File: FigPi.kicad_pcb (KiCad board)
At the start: 2 copper layers, 25.8 x 40.4 mm, 45 parts, among them J1 MOLEX_47346-100147346, J2 SPI0 / PWM2 / PWM3, J3 UART0 / PWM3 / PWM4, J4 STEMMA_1/QWIIC_1/I2C1/PMW1, J5 ADC / PWM5 / PWM6, J6 STEMMA_0/QWIIC_0/I2C0/PMW0, J7 PWR, SW1 KMS233GLFG, SW2 KMS233GLFG, U1 RP2040, U2 QSPI NOR FLASH 2MiB 2x3mm USO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, U3 AP2112K-3.3, U4 KC2520Z

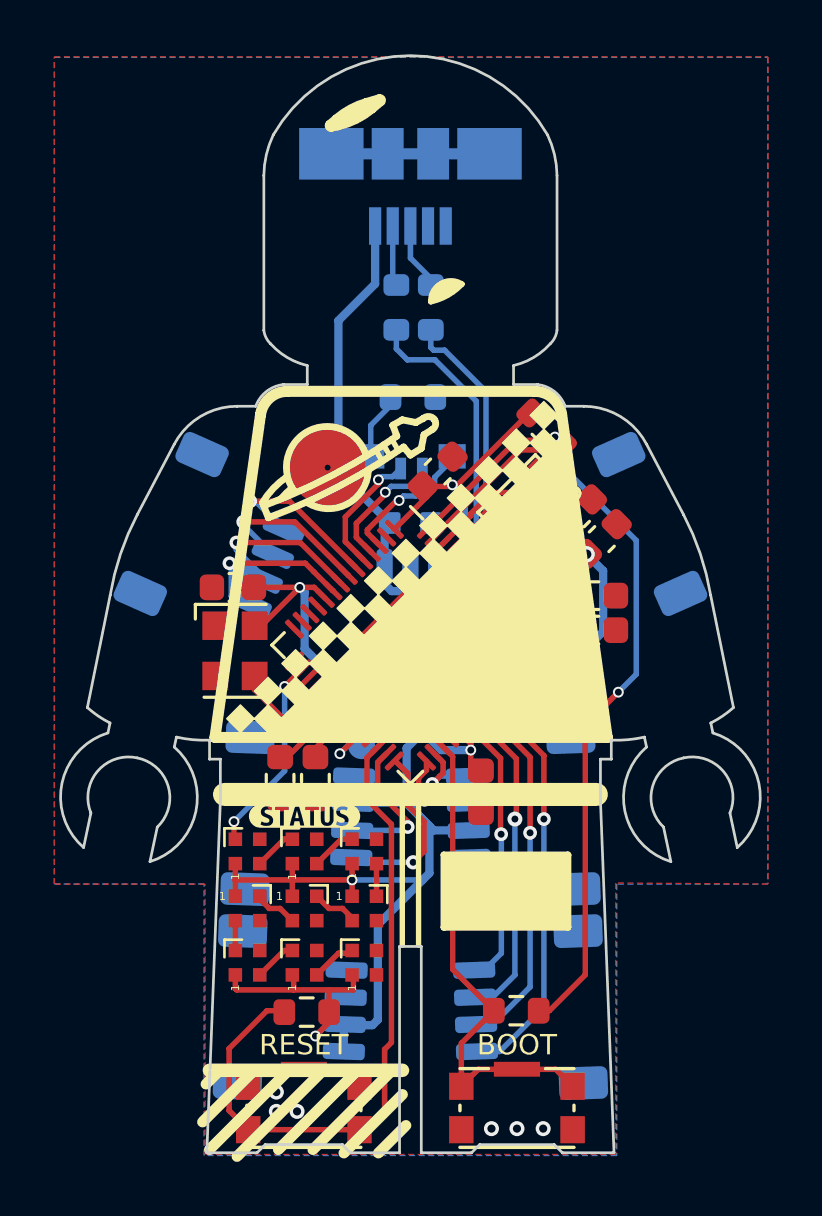
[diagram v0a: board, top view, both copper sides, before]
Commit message: 1.6 - Minor Cosmetic Changes
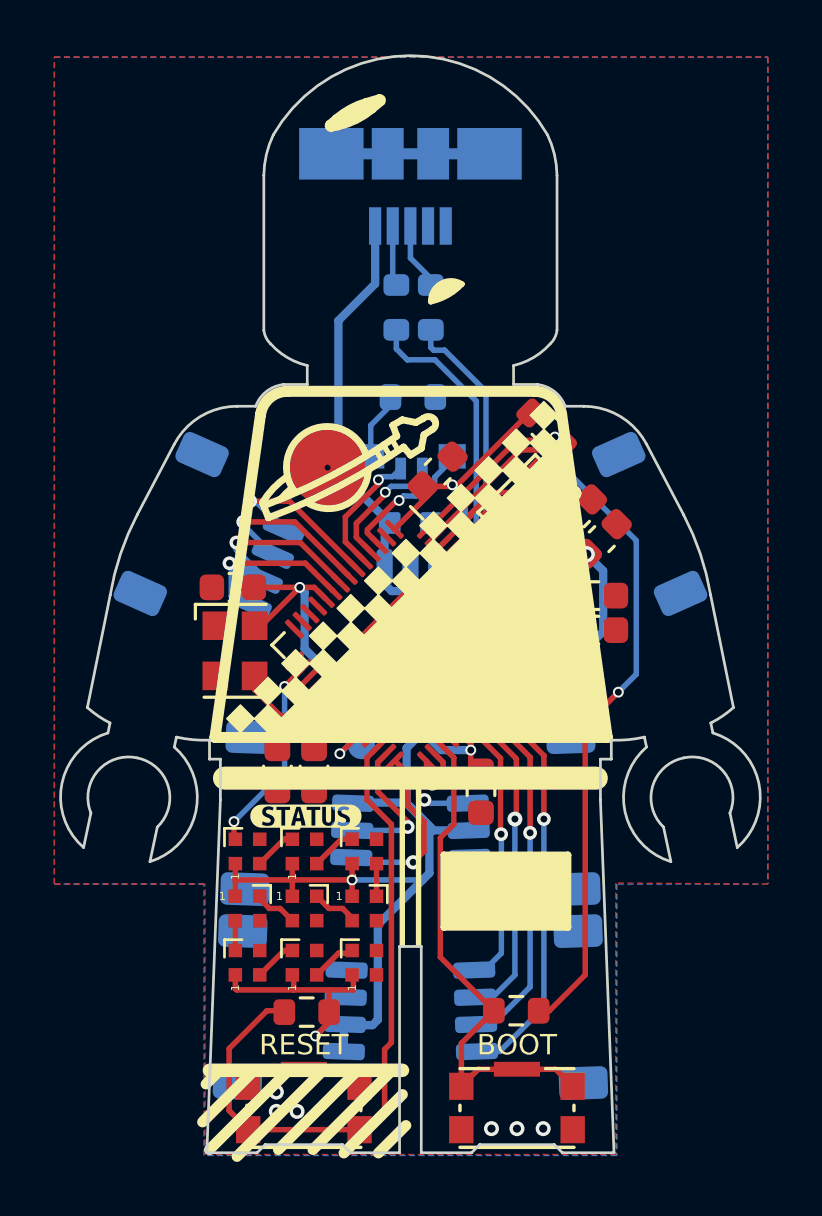
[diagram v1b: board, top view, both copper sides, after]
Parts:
- moved C8 0.32 mm to (7.10, -14.1)
- moved C3 0.30 mm to (8.45, -14.1)
- moved kibuzzard-620D4CA4 0.05 mm to (8.15, -12.4)
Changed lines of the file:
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@@
   )
   (footprint "Capacitor_SMD:C_0603_1608Metric" (layer "F.Cu")
-    (at 7.2 -13.8 90)
+    (at 7.1 -14.1 90)
     (descr "Capacitor SMD 0603 (1608 Metric), square (rectangular) end terminal, IPC_7351 nominal, (Body size source: IPC-SM-782 page 76, https://www.pcb-3d.com/wordpress/wp-content/uploads/ipc-sm-782a_amendment_1_and_2.pdf), generated with kicad-footprint-generator")
     (tags "capacitor")
@@
   )
   (footprint "Capacitor_SMD:C_0603_1608Metric" (layer "F.Cu")
-    (at 8.5 -13.8 90)
+    (at 8.45 -14.1 90)
     (descr "Capacitor SMD 0603 (1608 Metric), square (rectangular) end terminal, IPC_7351 nominal, (Body size source: IPC-SM-782 page 76, https://www.pcb-3d.com/wordpress/wp-content/uploads/ipc-sm-782a_amendment_1_and_2.pdf), generated with kicad-footprint-generator")
     (tags "capacitor")
@@
   )
   (footprint "kibuzzard-620D4CA4" (layer "F.Cu")
-    (at 8.1 -12.4)
+    (at 8.15 -12.4)
     (descr "Converted using: scripting")
     (tags "svg2mod")
@@
   (gr_line (start 11.7 -13.35) (end 11.7 -7.65) (layer "F.SilkS") (width 0.2))
   (gr_arc (start 6.478558 -27.189797) (mid 6.812918 -27.804917) (end 7.46874 -28.05) (layer "F.SilkS") (width 0.4064))
-  (gr_line (start 18.85 -13.2) (end 5.15 -13.2) (layer "F.SilkS") (width 0.85))
+  (gr_line (start 18.85 -13.8) (end 5.15 -13.8) (layer "F.SilkS") (width 0.85))
   (gr_line (start 16.581259 -28.05) (end 7.46874 -28.05) (layer "F.SilkS") (width 0.4064))
   (gr_arc (start 16.581257 -28.05) (mid 17.23708 -27.804917) (end 17.57144 -27.189796) (layer "F.SilkS") (width 0.4064))
@@
   (segment (start 5.55 -6.05) (end 5.55 -6.55) (width 0.2032) (layer "F.Cu") (net 3))
   (segment (start 18.021 -18.679) (end 18.021 -19.2532) (width 0.3048) (layer "F.Cu") (net 3))
+  (segment (start 7.1 -14.875) (end 7.925 -15.7) (width 0.2032) (layer "F.Cu") (net 3))
   (segment (start 9.0038 -5.9962) (end 9 -6) (width 0.2032) (layer "F.Cu") (net 3))
   (segment (start 18.3 -18.4) (end 18.177208 -18.277208) (width 0.3048) (layer "F.Cu") (net 3))
+  (segment (start 7.925 -15.7) (end 8.9 -15.7) (width 0.2032) (layer "F.Cu") (net 3))
   (segment (start 9.282843 -15.7) (end 9.710742 -16.127899) (width 0.2032) (layer "F.Cu") (net 3))
   (segment (start 18.021 -18.964616) (end 17.333592 -18.277208) (width 0.2032) (layer "F.Cu") (net 3))
-  (segment (start 8.9 -15.7) (end 8.591 -15.7) (width 0.2032) (layer "F.Cu") (net 3))
   (segment (start 18.021 -20.5232) (end 18.454002 -20.090198) (width 0.2032) (layer "F.Cu") (net 3))
   (segment (start 7.65 -10.15) (end 7.65 -10.75) (width 0.2032) (layer "F.Cu") (net 3))
@@
   (segment (start 9.9 -6.5) (end 9.9 -6) (width 0.2032) (layer "F.Cu") (net 3))
   (segment (start 17.500155 -20.5232) (end 18.021 -20.5232) (width 0.2032) (layer "F.Cu") (net 3))
-  (segment (start 8.591 -15.7) (end 7.493 -14.602) (width 0.2032) (layer "F.Cu") (net 3))
   (segment (start 17.075658 -22.005596) (end 18.249588 -22.005596) (width 0.2032) (layer "F.Cu") (net 3))
   (segment (start 15.986314 -19.575045) (end 16.269157 -19.292202) (width 0.2032) (layer "F.Cu") (net 3))
@@
   (segment (start 13.875 -2.45) (end 13.85 -2.45) (width 0.2032) (layer "F.Cu") (net 28))
   (segment (start 14.5 -3.075) (end 13.875 -2.45) (width 0.2032) (layer "F.Cu") (net 28))
-  (segment (start 13.559081 -6.748719) (end 15.0754 -5.2324) (width 0.2) (layer "F.Cu") (net 28))
+  (segment (start 13.1 -7.2078) (end 13.1 -11.6) (width 0.2) (layer "F.Cu") (net 28))
   (segment (start 15.925 -3.075) (end 17.35 -3.075) (width 0.2032) (layer "F.Cu") (net 28))
   (segment (start 17.35 -3.075) (end 17.975 -2.45) (width 0.2032) (layer "F.Cu") (net 28))
-  (segment (start 13.559081 -14.595334) (end 13.559081 -6.748719) (width 0.2) (layer "F.Cu") (net 28))
+  (segment (start 13.1 -11.6) (end 13.6 -12.1) (width 0.2) (layer "F.Cu") (net 28))
+  (segment (start 15.0754 -5.2324) (end 13.1 -7.2078) (width 0.2) (layer "F.Cu") (net 28))
   (segment (start 13.875 -4.032) (end 15.0754 -5.2324) (width 0.2032) (layer "F.Cu") (net 28))
-  (segment (start 13.157887 -14.996528) (end 13.559081 -14.595334) (width 0.2) (layer "F.Cu") (net 28))
+  (segment (start 13.6 -12.1) (end 13.6 -14.554415) (width 0.2) (layer "F.Cu") (net 28))
+  (segment (start 13.6 -14.554415) (end 13.157887 -14.996528) (width 0.2) (layer "F.Cu") (net 28))
   (segment (start 13.875 -2.45) (end 13.875 -4.032) (width 0.2032) (layer "F.Cu") (net 28))
   (segment (start 17.907 -2.518) (end 17.975 -2.45) (width 0.2032) (layer "F.Cu") (net 28))
@@
   (segment (start 10.935599 -24.905599) (end 11.341199 -24.905599) (width 0.2032) (layer "B.Cu") (net 35))
   (segment (start 11.341199 -24.905599) (end 11.6396 -25.204) (width 0.2032) (layer "B.Cu") (net 35))
+  (segment (start 7.2172 -16.1) (end 6.2622 -17.055) (width 0.2032) (layer "F.Cu") (net 36))
+  (segment (start 8.551471 -16.1) (end 7.2172 -16.1) (width 0.2032) (layer "F.Cu") (net 36))
   (segment (start 6.2622 -17.055) (end 6.2622 -17.5662) (width 0.2032) (layer "F.Cu") (net 36))
-  (segment (start 8.504271 -16.0528) (end 7.2644 -16.0528) (width 0.2032) (layer "F.Cu") (net 36))
-  (segment (start 9.145056 -16.693585) (end 8.504271 -16.0528) (width 0.2032) (layer "F.Cu") (net 36))
-  (segment (start 7.2644 -16.0528) (end 6.2622 -17.055) (width 0.2032) (layer "F.Cu") (net 36))
+  (segment (start 9.145056 -16.693585) (end 8.551471 -16.1) (width 0.2032) (layer "F.Cu") (net 36))
   (segment (start 15.321099 -14.530372) (end 15.321099 -11.755301) (width 0.2032) (layer "F.Cu") (net 39))
   (segment (start 15.321099 -11.755301) (end 15.3416 -11.7348) (width 0.2032) (layer "F.Cu") (net 39))
